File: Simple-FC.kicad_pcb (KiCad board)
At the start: 2 copper layers, 40 x 40 mm, 76 parts, among them J1 USB_C_Receptacle_USB2.0_14P, J10 Conn_01x01, J2 Micro_SD_Card, J3 Conn_01x04, J4 Conn_01x04, J5 Conn_01x04, J6 Conn_01x05, J7 Conn_01x04, J8 Conn_01x03, J9 Conn_01x01, SW1 SW_Push, U1 RP2350A, U2 MMC5983MA, U3 LSM6DSM, U4 BMP384, U5 TPS631000, U6 W25Q128JVS, Y1 ABM8-272-T3

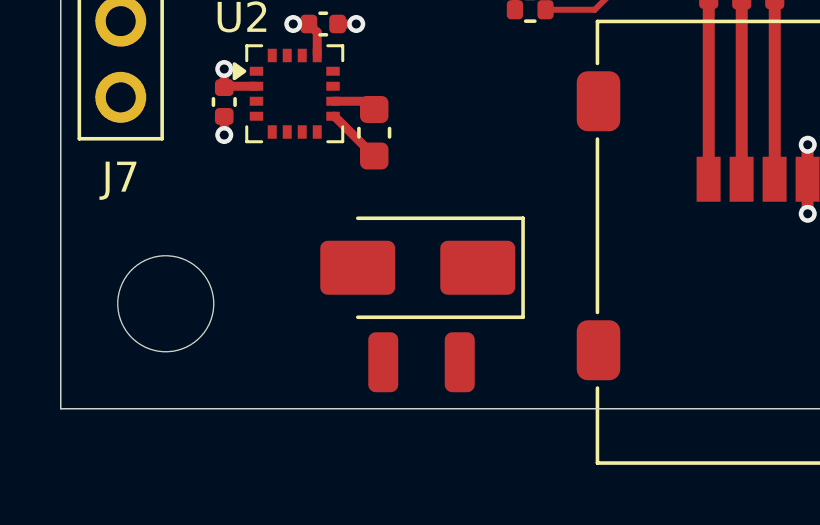
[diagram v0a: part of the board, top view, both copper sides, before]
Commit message: added power trace
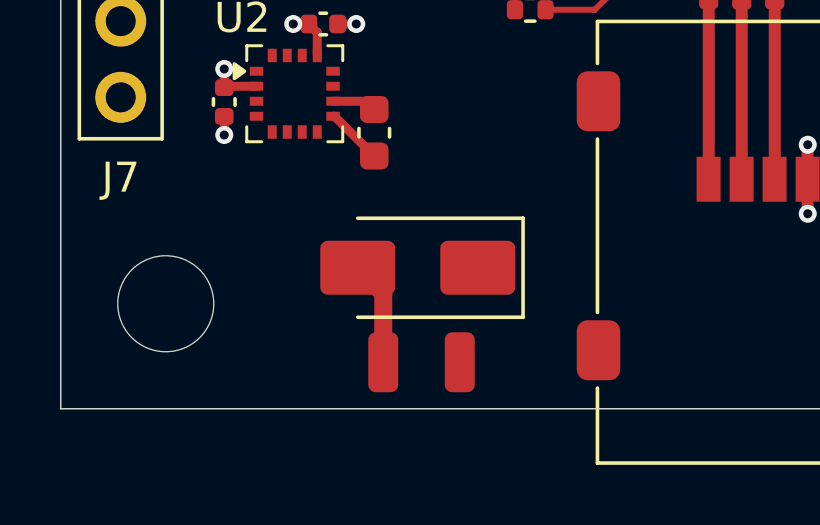
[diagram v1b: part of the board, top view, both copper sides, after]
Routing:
- net Net-(D2-A): track 0.00 -> 3.50 mm
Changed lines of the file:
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@@
+	)
+	(segment
+		(start 135.75 123.45)
+		(end 135.75 121.15)
+		(width 0.6)
+		(layer "F.Cu")
+		(net "Net-(D2-A)")
+	)
+	(segment
+		(start 135.75 121.15)
+		(end 134.9 120.3)
+		(width 0.6)
+		(layer "F.Cu")
+		(net "Net-(D2-A)")
 	)
 	(segment
